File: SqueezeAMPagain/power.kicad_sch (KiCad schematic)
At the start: 45 parts, among them J6 Conn_01x02_Pin, J7 Barrel_Jack_Switch_MountingPin, Q1 Q_NPN_BEC, Q2 PMOS, Q3 PMOS, Q6 Q_NPN_BEC, Q7 PMOS, U5 TPS5430DDA

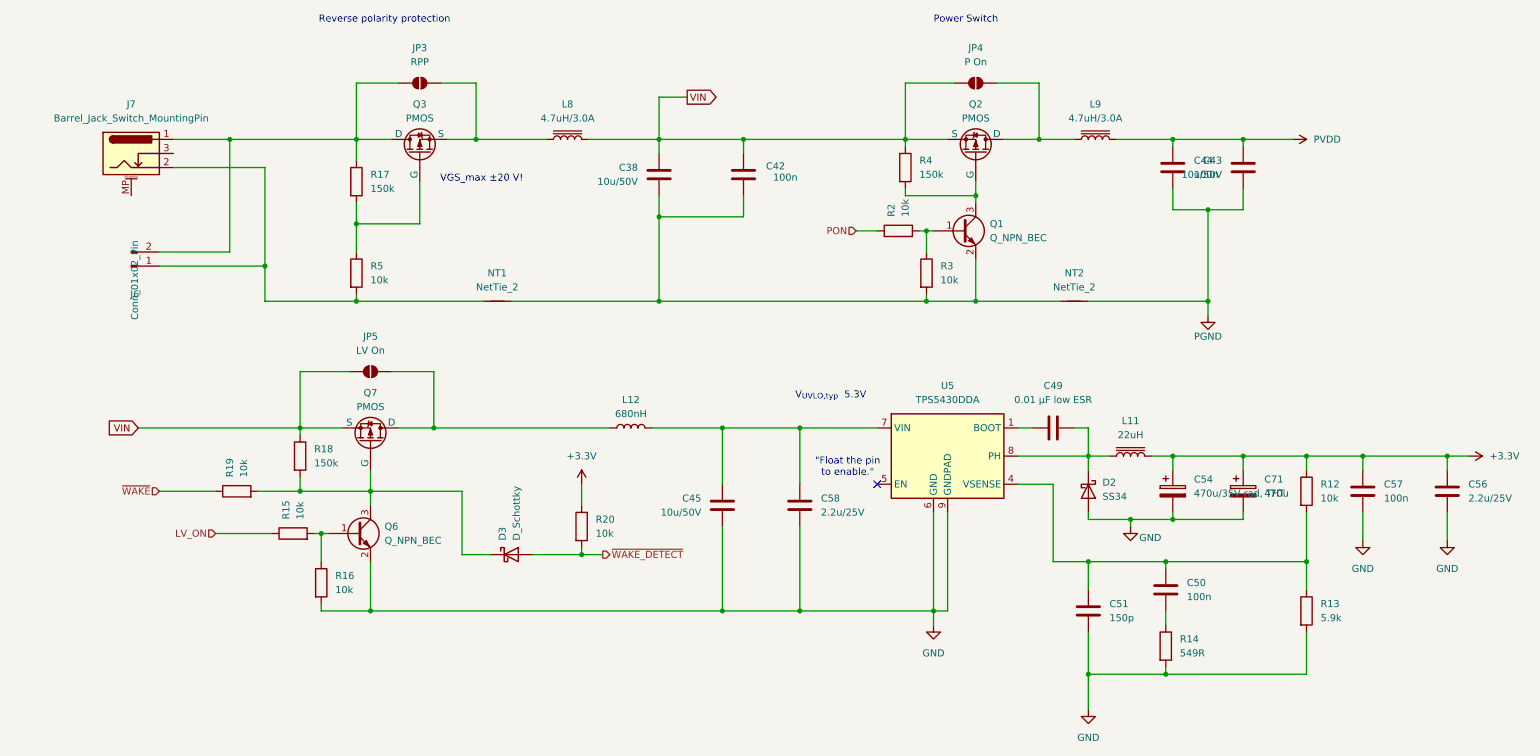
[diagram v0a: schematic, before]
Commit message: Update SqueezeAMPagain.kicad_pcb, SqueezeAMPagain.kicad_prl, USB-Uart.kicad_sch, and 4 more files
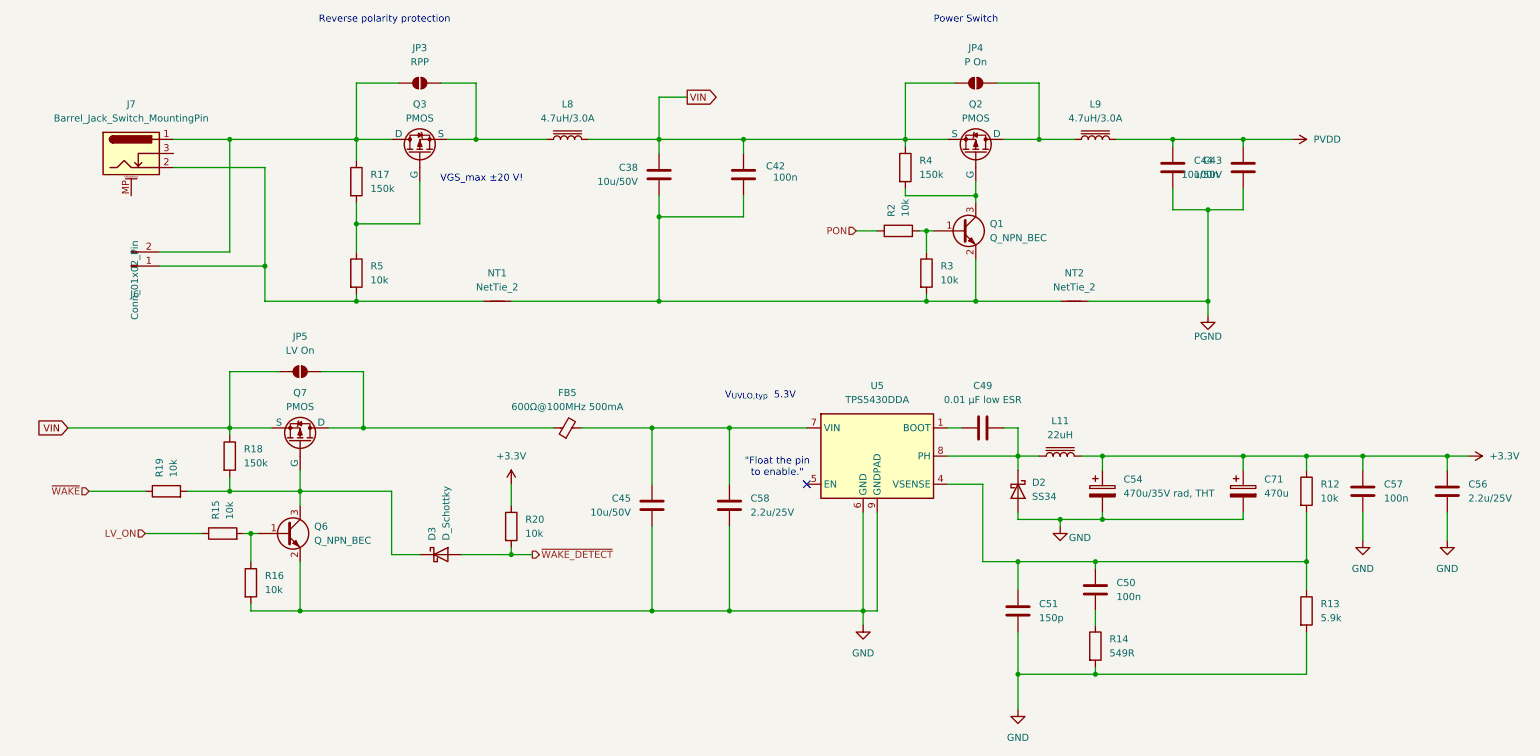
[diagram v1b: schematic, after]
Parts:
- removed L12: 680nH, Inductor_SMD:L_0805_2012Metric, symbol Device:L
- added FB5: 600Ω@100MHz 500mA, Inductor_SMD:L_0805_2012Metric, symbol Device:FerriteBead_Small
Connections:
- net at C45.1, C58.1, U5.7 (VIN): now also FB5.2
- net at JP5.2 (B), Q7.1 (D): now also FB5.1
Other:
- moved on the sheet: C45, C49, C50, C51, C54, C58, D2, D3, JP5, L11, Q6, Q7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

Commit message: Update SqueezeAMPagain.kicad_pcb, project.db, power.kicad_sch, and 1 more file
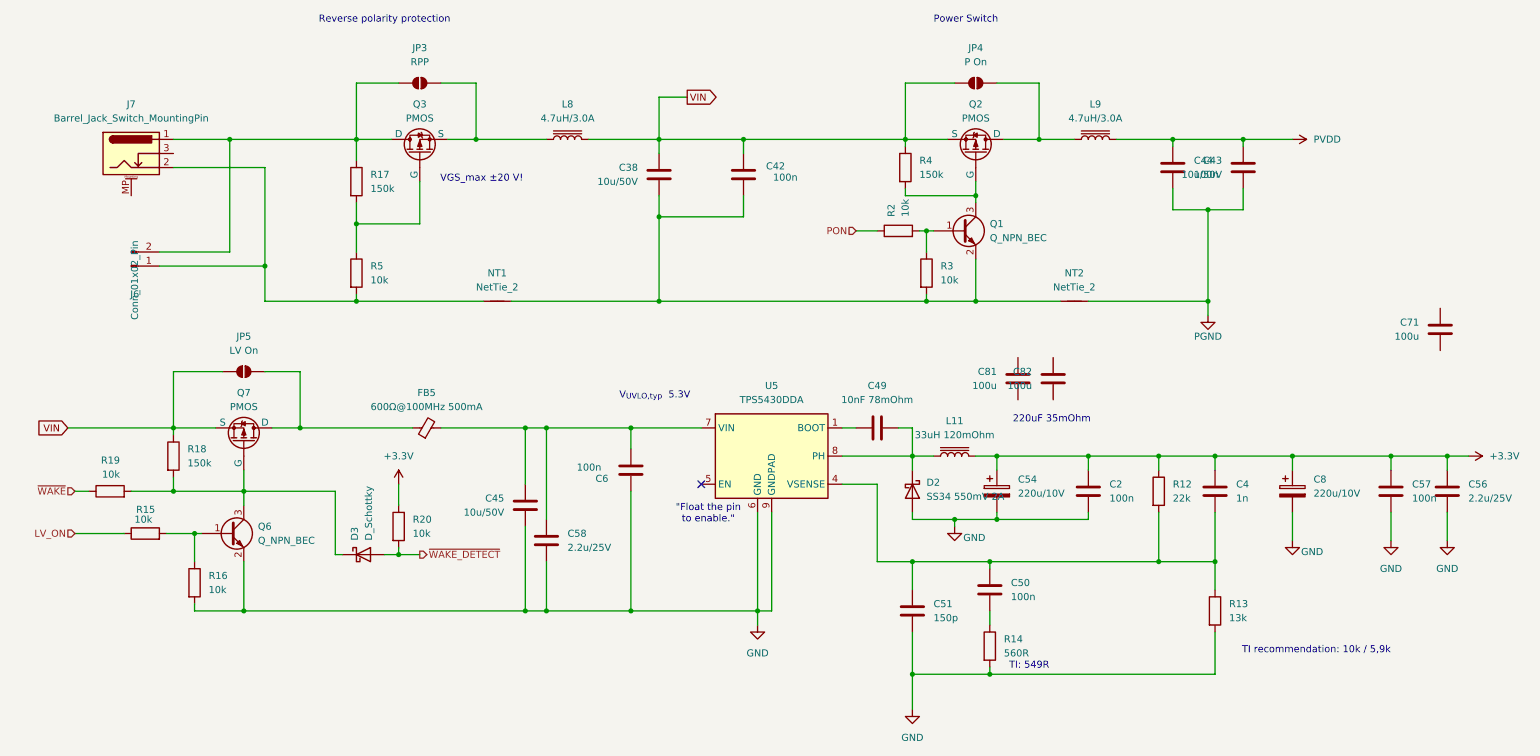
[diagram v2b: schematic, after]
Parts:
- removed C71: 470u, Capacitor_SMD:CP_Elec_6.3x3.9, symbol Device:C_Polarized
- added C2, C6: 100n, Capacitor_SMD:C_0603_1608Metric, symbol Device:C
- added C4: 1n, Capacitor_SMD:C_0603_1608Metric, symbol Device:C
- added C71, C81, C82: 100u, Capacitor_SMD:C_1206_3216Metric, symbol Device:C
- added C8: 220u/10V, Capacitor_THT:CP_Radial_D10.0mm_P2.50mm_P5.00mm, symbol Device:C_Polarized
- C49: value 0.01 μF low ESR -> 10nF 78mOhm
- C54: value 470u/35V rad, THT -> 220u/10V; footprint Capacitor_THT:CP_Radial_D8.0mm_P5.00mm -> Capacitor_THT:CP_Radial_D10.0mm_P2.50mm_P5.00mm; mfr# (none) -> EEUFR1A221; reichelt FR-A 470U 35-3 -> FR-A 220U 10 / FR-A 220U 10B
- C58: footprint Capacitor_SMD:C_0603_1608Metric -> Capacitor_SMD:C_0805_2012Metric
- D2: value SS34 -> SS34 550mV 2A
- L11: value 22uH -> 33uH 120mOhm
- R12: value 10k -> 22k
- R13: value 5.9k -> 13k
- R14: value 549R -> 560R
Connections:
- net +3.3V: now also C2.1, C4.1, C8.1
- net GND: now also C2.2, C6.1, C8.2
- net at C45.1, C58.1, FB5.2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: now also C6.2
- net at C50.1, C51.1, R12.2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: now also C4.2
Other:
- note added: "220uF 35mOhm"
- note added: "TI recommendation: 10k / 5,9k"
- note added: "TI: 549R"
- moved on the sheet: C45, C49, C50, C51, C54, C57, C58, D2, D3, FB5, JP5, L11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
